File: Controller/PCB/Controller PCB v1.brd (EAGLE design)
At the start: 100 x 80 mm, 7 parts, among them IC1 74HC4051N,652, IC2 74HC4051N,652

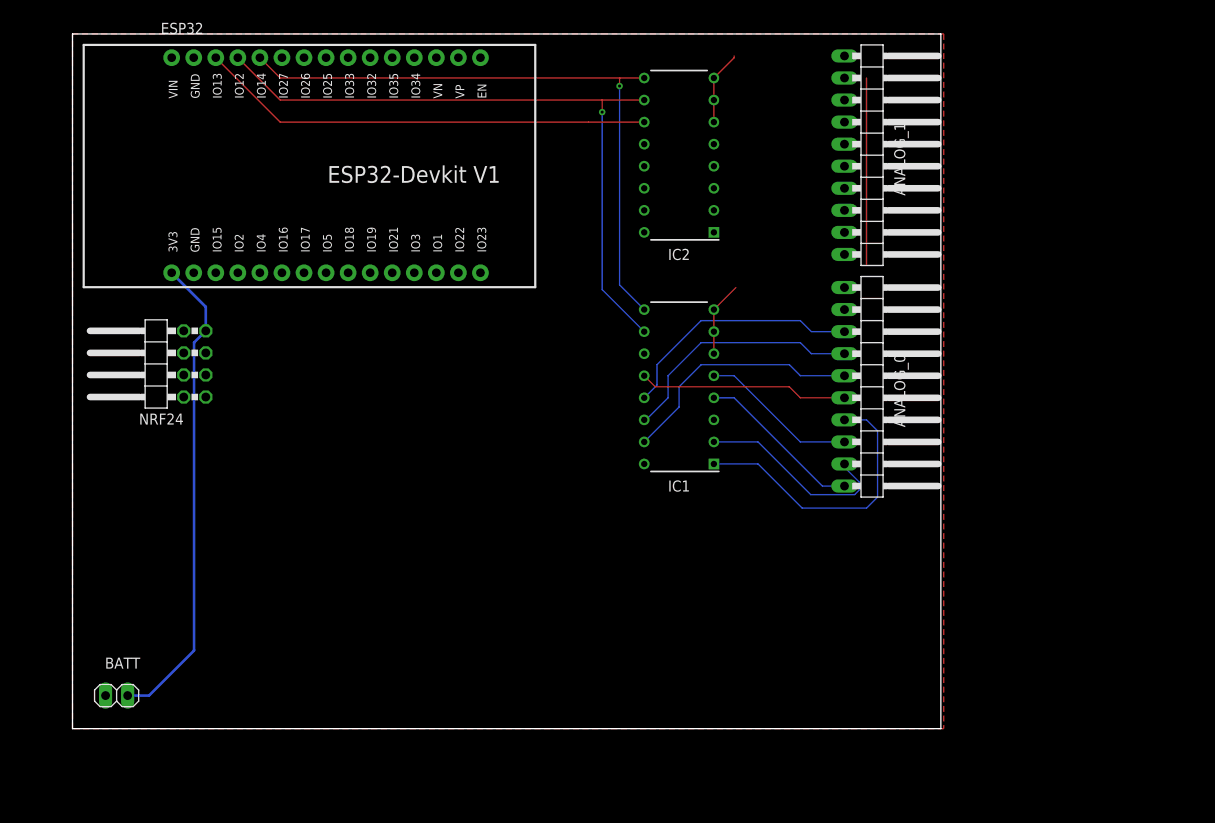
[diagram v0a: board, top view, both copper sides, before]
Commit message: pcb work
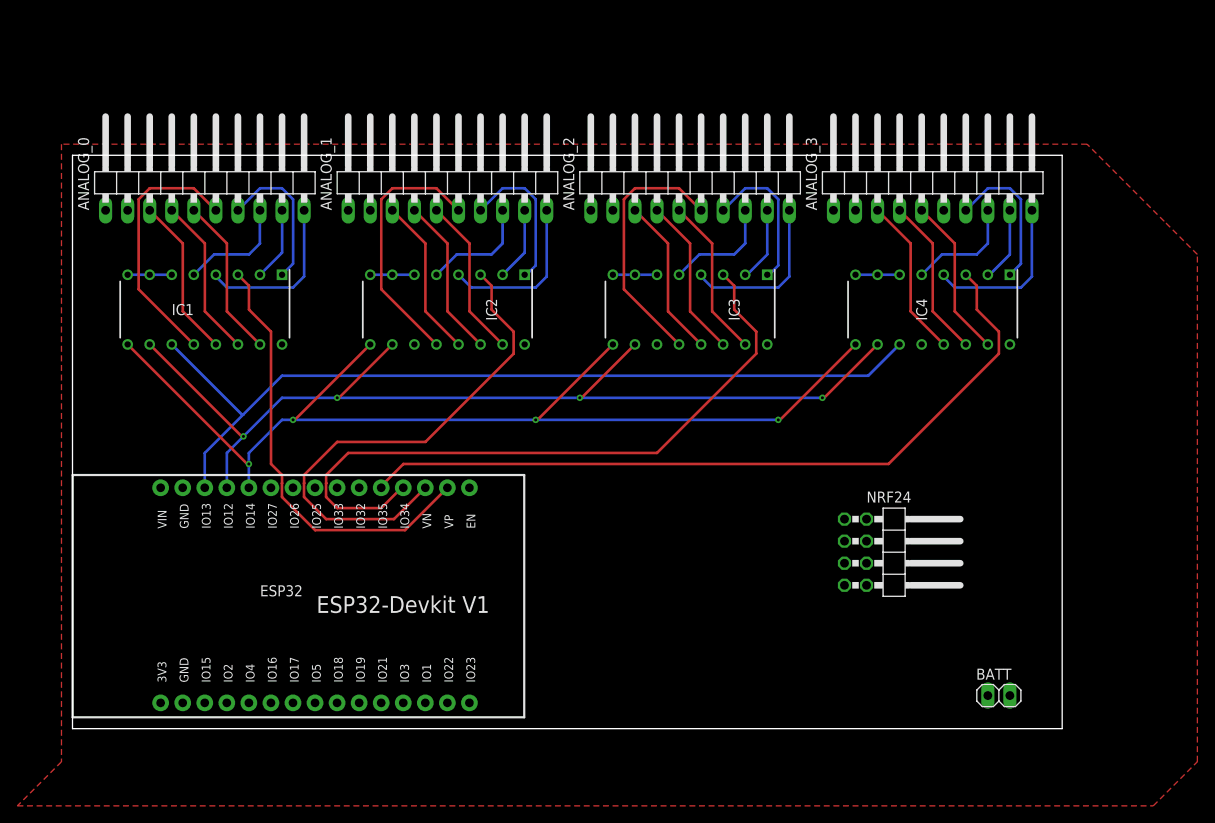
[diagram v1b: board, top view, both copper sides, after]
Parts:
- added ANALOG_2, ANALOG_3: (no value), pinhead:1X10/90
- added IC3, IC4: 74HC4051N,652, 74HC4051N_652:DIP802W53P254L1902H420Q16N
- moved BATT 101.6 mm to (106.7, 3.81)
- moved NRF24 88.9 mm to (95.2, 20.3), turned to 270 degrees
- moved ANALOG_0 81.1 mm to (15.2, 63.5), turned to 0 degrees
- moved IC1 55.3 mm to (15.2, 48.3), turned to 270 degrees
- moved ANALOG_1 49.6 mm to (43.2, 63.5), turned to 0 degrees
- moved ESP32 49.5 mm to (33.0, 16.5)
- moved IC2 32.1 mm to (43.2, 48.3), turned to 270 degrees
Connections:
- new net Y2_0: ANALOG_2.3, IC3.13
- new net Y2_1: ANALOG_2.4, IC3.14
- new net Y2_2: ANALOG_2.5, IC3.15
- new net Y2_3: ANALOG_2.6, IC3.12
- new net Y2_4: ANALOG_2.7, IC3.1
- new net Y2_5: ANALOG_2.8, IC3.5
- new net Y2_6: ANALOG_2.9, IC3.2
- new net Y2_7: ANALOG_2.10, IC3.4
- new net Y2_Z: ESP32.19, IC3.3
- new net Y3_0: ANALOG_3.3, IC4.13
- new net Y3_1: ANALOG_3.4, IC4.14
- new net Y3_2: ANALOG_3.5, IC4.15
- new net Y3_3: ANALOG_3.6, IC4.12
- new net Y3_4: ANALOG_3.7, IC4.1
- new net Y3_5: ANALOG_3.8, IC4.5
- new net Y3_6: ANALOG_3.9, IC4.2
- new net Y3_7: ANALOG_3.10, IC4.4
- new net Y3_Z: ESP32.20, IC4.3
- net +3V3: now also ANALOG_2.2, ANALOG_3.2, IC3.16, IC4.16
- net GND: now also ANALOG_2.1, ANALOG_3.1, IC3.6, IC3.7, IC3.8, IC4.6, IC4.7, IC4.8
- net S_0: now also IC3.11, IC4.11
- net S_1: now also IC3.10, IC4.10
- net S_2: now also IC3.9, IC4.9
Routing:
- net Y3_Z: track 0.00 -> 88.3 mm
- net Y2_Z: track 0.00 -> 78.9 mm
- net Y1_Z: track 0.00 -> 59.6 mm
- net +3V3: track 55.5 -> 0.00 mm
- net S_2: track 73.1 -> 123.7 mm, vias 1 -> 4
- net Y0_Z: track 0.00 -> 50.4 mm
- net S_0: track 52.4 -> 100.8 mm
- net S_1: track 77.5 -> 117.1 mm, vias 1 -> 4
- net Y2_3: track 0.00 -> 29.8 mm
- net Y1_3: track 0.00 -> 29.8 mm
- net Y3_7: track 0.00 -> 19.0 mm
- net Y2_7: track 0.00 -> 19.0 mm
- net Y1_7: track 0.00 -> 18.9 mm
- net Y3_1: track 0.00 -> 18.6 mm
- net Y3_0: track 0.00 -> 18.6 mm
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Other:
- board size 100 x 80 mm -> 114 x 66 mm
